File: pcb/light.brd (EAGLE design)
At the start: 13 x 13 mm, 5 parts, among them J3 FFC3B07-05-T, U1 TEMT6000

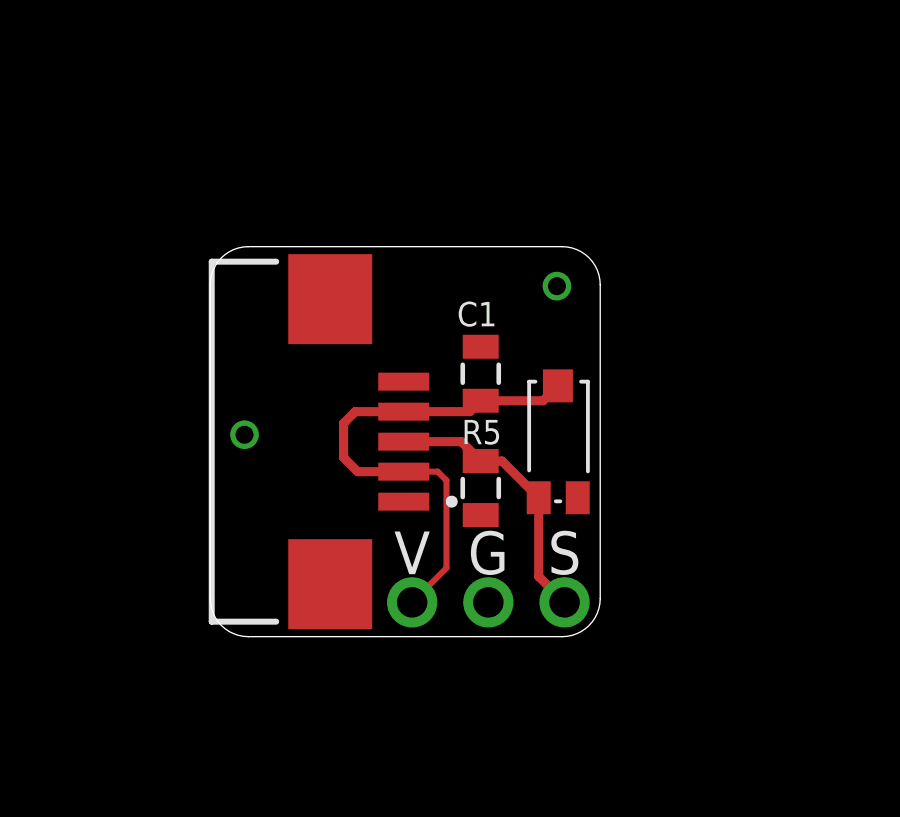
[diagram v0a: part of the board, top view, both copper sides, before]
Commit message: cleanup PCB files
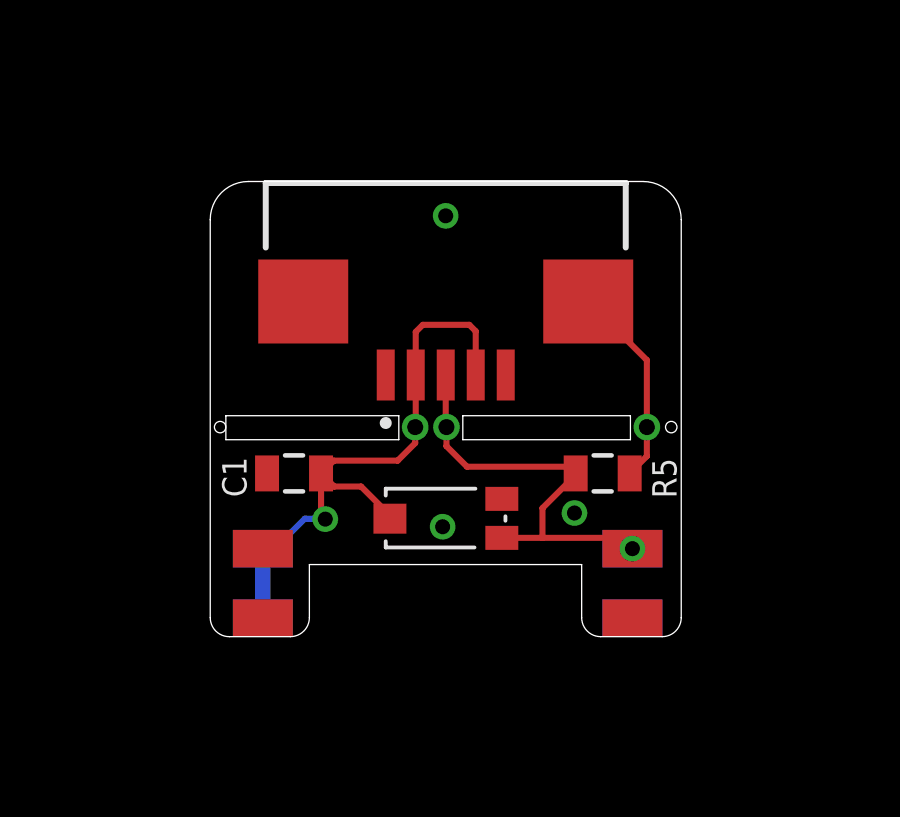
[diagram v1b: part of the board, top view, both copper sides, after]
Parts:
- removed JP1: (no value), adafruit_changed:1X03-CLEANBIG
- added U$1: LS_VERT, apricot:LS_VERT
- moved C1 7.05 mm to (2.79, 5.44), turned to 0 degrees
- moved J3 6.05 mm to (7.85, 11.2), turned to 180 degrees
- moved U1 4.54 mm to (7.85, 3.94), turned to 180 degrees
- moved R5 4.09 mm to (13.1, 5.44), turned to 180 degrees
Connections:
- net +3V3: now also U$1.B1, U$1.B2; no longer JP1.1
- net GND: now also U$1.T1, U$1.T2; no longer JP1.2
- net S: now also U$1.B3, U$1.B4, U$1.T3, U$1.T4; no longer JP1.3
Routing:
- net GND: track 0.00 -> 6.78 mm, vias 2 -> 4
- net S: track 9.12 -> 14.4 mm, vias 0 -> 2
- net +3V3: track 17.1 -> 20.3 mm, vias 0 -> 2
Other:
- board size 13 x 13 mm -> 15.7 x 15.2 mm
- board text added: "PulseHPT.com"
- board text removed: "G"
- board text removed: "PulseHPT.com dekuNukem 2023"
- board text removed: "S"
- board text removed: "V"
